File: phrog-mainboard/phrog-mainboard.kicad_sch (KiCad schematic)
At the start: 52 parts, among them J1 Battery, Q1 2N7000, Q2 2N7000, SW1 SW_Push, SW3 SW_SPDT, U1 NRF52840 Pro Micro, U2 LM358, U3 NAU7802KGI, U4 MCP34063

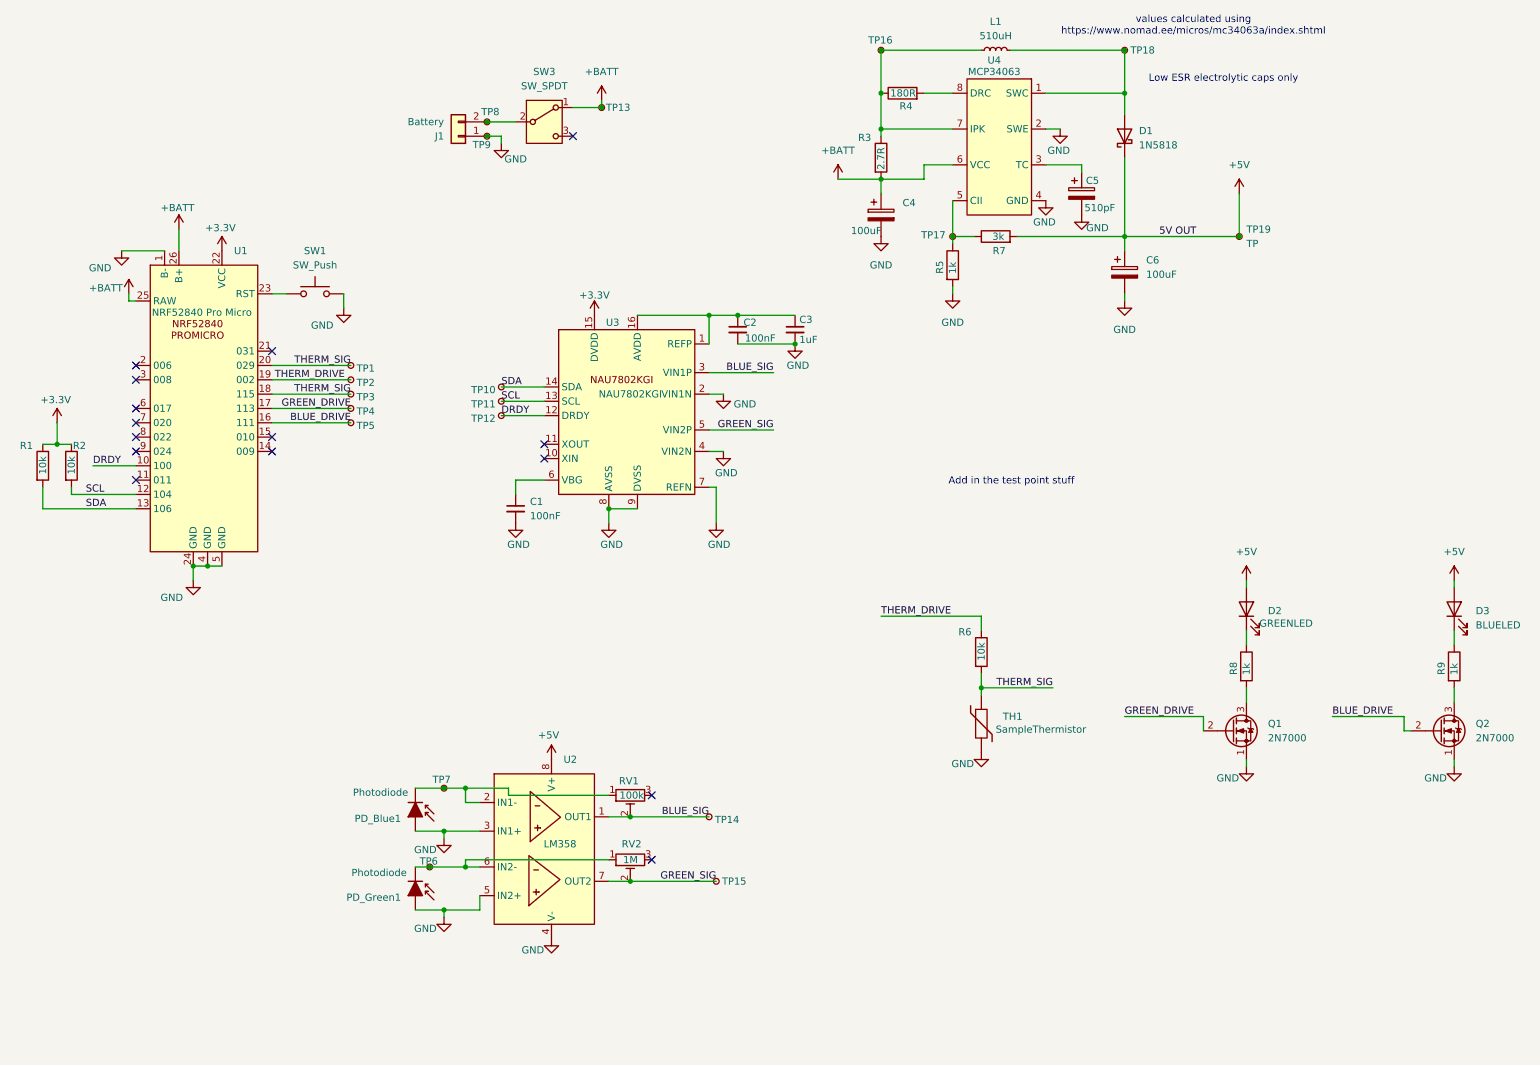
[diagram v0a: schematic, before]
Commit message: finish first draft of enclosure
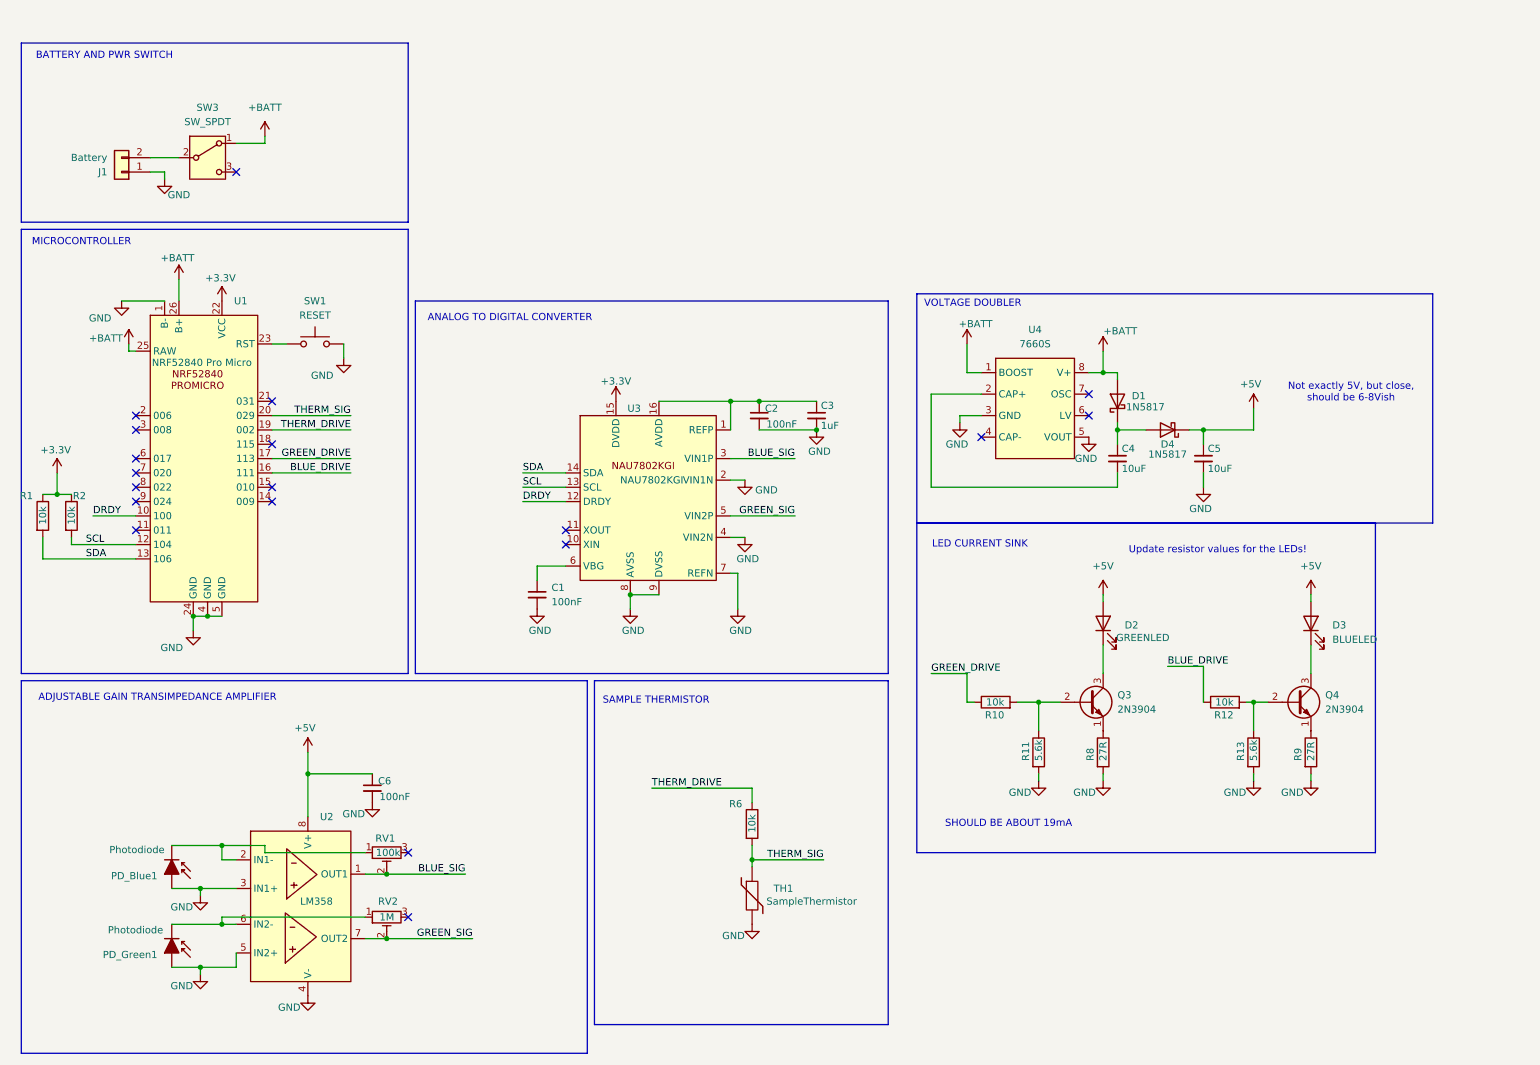
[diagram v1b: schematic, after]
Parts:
- removed C4, C6: 100uF, Capacitor_THT:CP_Radial_D8.0mm_P5.00mm, symbol Device:C_Polarized
- removed C5: 510pF, Capacitor_THT:C_Disc_D4.3mm_W1.9mm_P5.00mm, symbol Device:C_Polarized
- removed D1: 1N5818, Diode_THT:D_DO-41_SOD81_P10.16mm_Horizontal, symbol Diode:1N5818
- removed L1: 510uH, Inductor_THT:L_Axial_L11.0mm_D4.5mm_P15.24mm_Horizontal_Fastron_MECC, symbol Device:L_Small
- removed Q1, Q2: 2N7000, Package_TO_SOT_THT:TO-92_Inline, symbol Transistor_FET:2N7000
- removed R3: 2.7R, Resistor_THT:R_Axial_DIN0207_L6.3mm_D2.5mm_P10.16mm_Horizontal, symbol Device:R
- removed R4: 180R, Resistor_THT:R_Axial_DIN0207_L6.3mm_D2.5mm_P10.16mm_Horizontal, symbol Device:R
- removed R5: 1k, Resistor_THT:R_Axial_DIN0207_L6.3mm_D2.5mm_P10.16mm_Horizontal, symbol Device:R
- removed R7: 3k, Resistor_THT:R_Axial_DIN0207_L6.3mm_D2.5mm_P10.16mm_Horizontal, symbol Device:R
- removed TP1, TP10, TP11, TP12, TP13, TP14, TP15, TP16, TP17, TP18, TP19, TP2, TP3, TP4, TP5, TP6, TP7, TP8, TP9: TP, TestPoint:TestPoint_THTPad_D2.0mm_Drill1.0mm, symbol Connector:TestPoint_Small
- removed U4: MCP34063, Package_DIP:DIP-8_W7.62mm_LongPads, symbol -project:MCP34063
- added C4, C5: 10uF, Capacitor_THT:C_Disc_D4.3mm_W1.9mm_P5.00mm, symbol Device:C_Small
- added C6: 100nF, Capacitor_THT:C_Disc_D4.3mm_W1.9mm_P5.00mm, symbol Device:C_Small
- added D1, D4: 1N5817, Diode_THT:D_DO-41_SOD81_P10.16mm_Horizontal, symbol Diode:1N5817
- added Q3, Q4: 2N3904, Package_TO_SOT_THT:TO-92_Inline, symbol Transistor_BJT:2N3904
- added R10, R12: 10k, Resistor_THT:R_Axial_DIN0207_L6.3mm_D2.5mm_P10.16mm_Horizontal, symbol Device:R
- added R11, R13: 5.6k, Resistor_THT:R_Axial_DIN0207_L6.3mm_D2.5mm_P10.16mm_Horizontal, symbol Device:R
- added U4: 7660S, Package_DIP:DIP-8_W7.62mm_LongPads, symbol -project:7660S
- R8, R9: value 1k -> 27R
- SW1: value SW_Push -> RESET
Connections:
- net +5V: now also C5.1, C6.1, D4.1 (K)
- net +BATT: now also D1.2 (A), U4.1 (BOOST), U4.8 (V+)
- net BLUE_DRIVE: now also R12.1
- net GND: now also R8.2, R9.2, C5.2, C6.2, R11.2, R13.2, U4.3 (GND), U4.5 (VOUT)
- net GREEN_DRIVE: now also R10.1
- net THERM_SIG: no longer U1.18 (115)
- net at D2.1 (K): now also Q3.3 (C); no longer R8.1
- net at R9.1: now also Q4.1 (E); no longer D3.1 (K)
- new net: Q4.2 (B), R12.2, R13.1
- new net: Q3.2 (B), R10.2, R11.1
- new net: D3.1 (K), Q4.3 (C)
- new net: C4.2, U4.2 (CAP+)
- new net: C4.1, D1.1 (K), D4.2 (A)
- new net: Q3.1 (E), R8.1
- no-connect marks 15 -> 19
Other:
- note added: "ADJUSTABLE GAIN TRANSIMPEDANCE AMPLIFIER"
- note added: "ANALOG TO DIGITAL CONVERTER"
- note added: "BATTERY AND PWR SWITCH"
- note added: "LED CURRENT SINK"
- note added: "MICROCONTROLLER"
- note added: "Not exactly 5V, but close, should be 6-8Vish"
- note added: "SAMPLE THERMISTOR"
- note added: "SHOULD BE ABOUT 19mA"
- note added: "Update resistor values for the LEDs!"
- note added: "VOLTAGE DOUBLER"
- note removed: "Add in the test point stuff"
- note removed: "Low ESR electrolytic caps only"
- note removed: "values calculated using https://www.nomad.ee/micros/mc34063a/index.shtml"
- moved on the sheet: C1, C2, C3, D2, D3, J1, PD_Blue1, PD_Green1, R1, R2, R6, R8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
